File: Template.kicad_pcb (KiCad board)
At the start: 2 copper layers, 70 x 70 mm, 5 parts, among them J1 Conn_02x10_Odd_Even, J2 Conn_01x08, J3 Conn_01x08

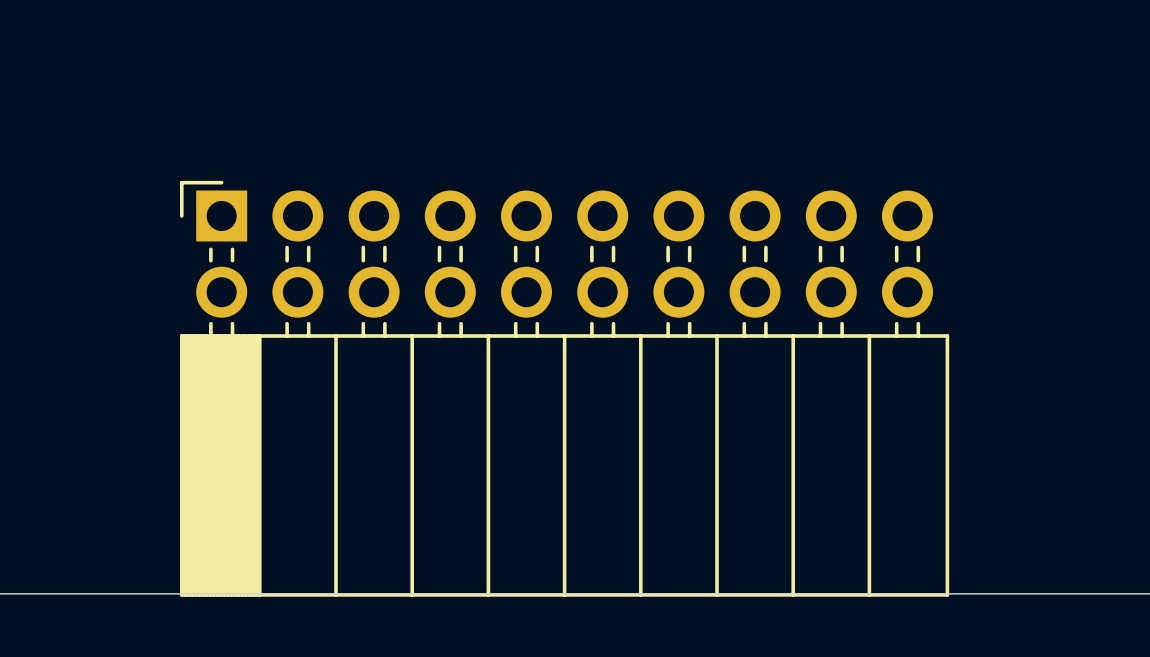
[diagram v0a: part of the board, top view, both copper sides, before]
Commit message: Small edit
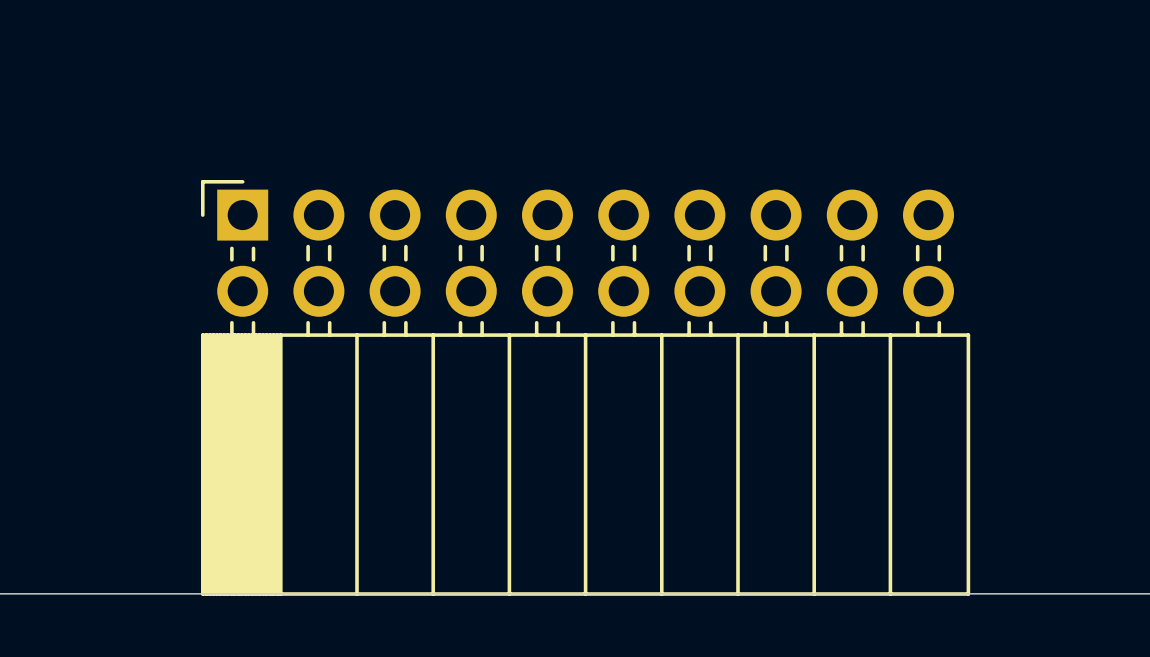
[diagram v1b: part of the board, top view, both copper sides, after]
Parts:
- moved J1 0.70 mm to (103.5, 107.4)
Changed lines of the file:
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@@
   )
   (footprint "Connector_PinSocket_2.54mm:PinSocket_2x10_P2.54mm_Horizontal" (layer "F.Cu")
-    (at 102.85 107.405 90)
+    (at 103.55 107.375 90)
     (descr "Through hole angled socket strip, 2x10, 2.54mm pitch, 8.51mm socket length, double cols (from Kicad 4.0.7), script generated")
     (tags "Through hole angled socket strip THT 2x10 2.54mm double row")
